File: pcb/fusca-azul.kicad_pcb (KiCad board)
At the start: 2 copper layers, 59 x 67.5 mm, 12 parts, among them J3 HC-SR04, J4 L298N Logic Jumpers, J5 HC-SR04, J6 HC-SR04, U2 ESP32 - HW-394

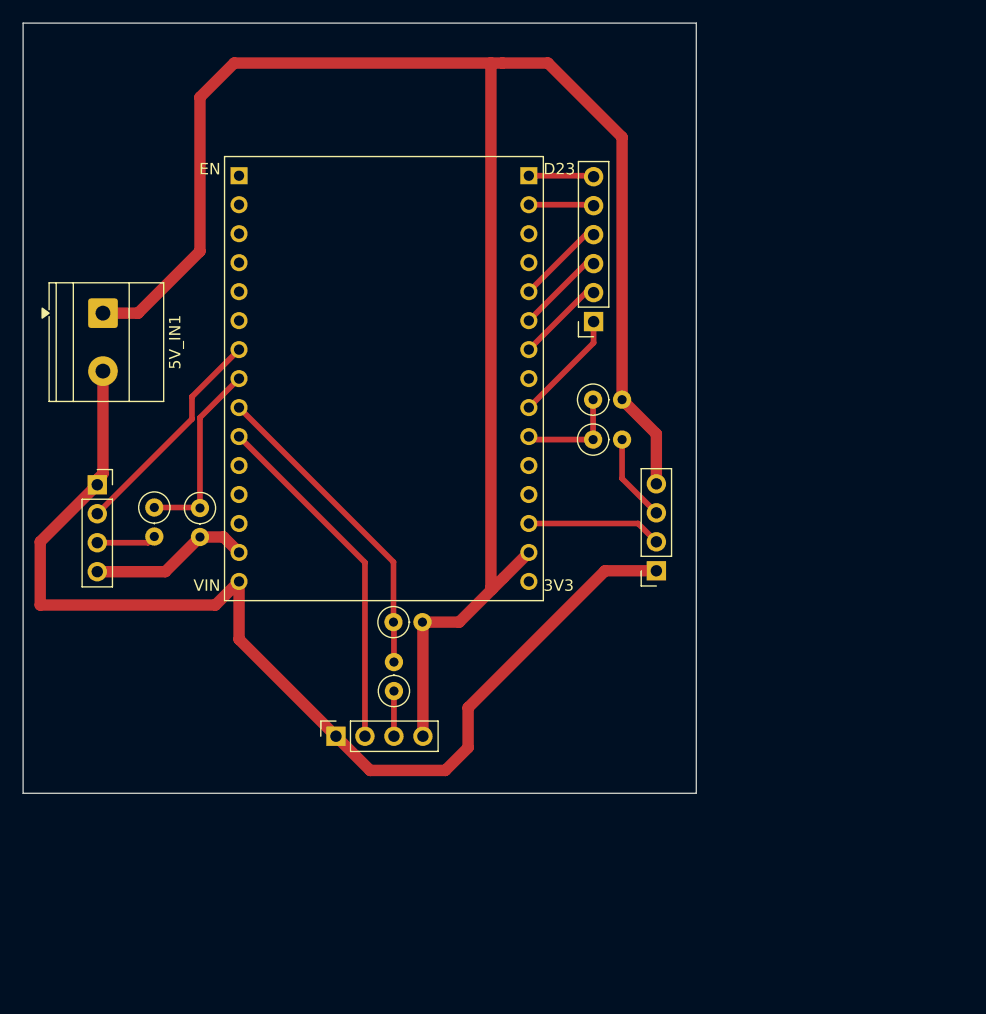
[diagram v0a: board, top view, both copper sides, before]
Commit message: finaliza pcb
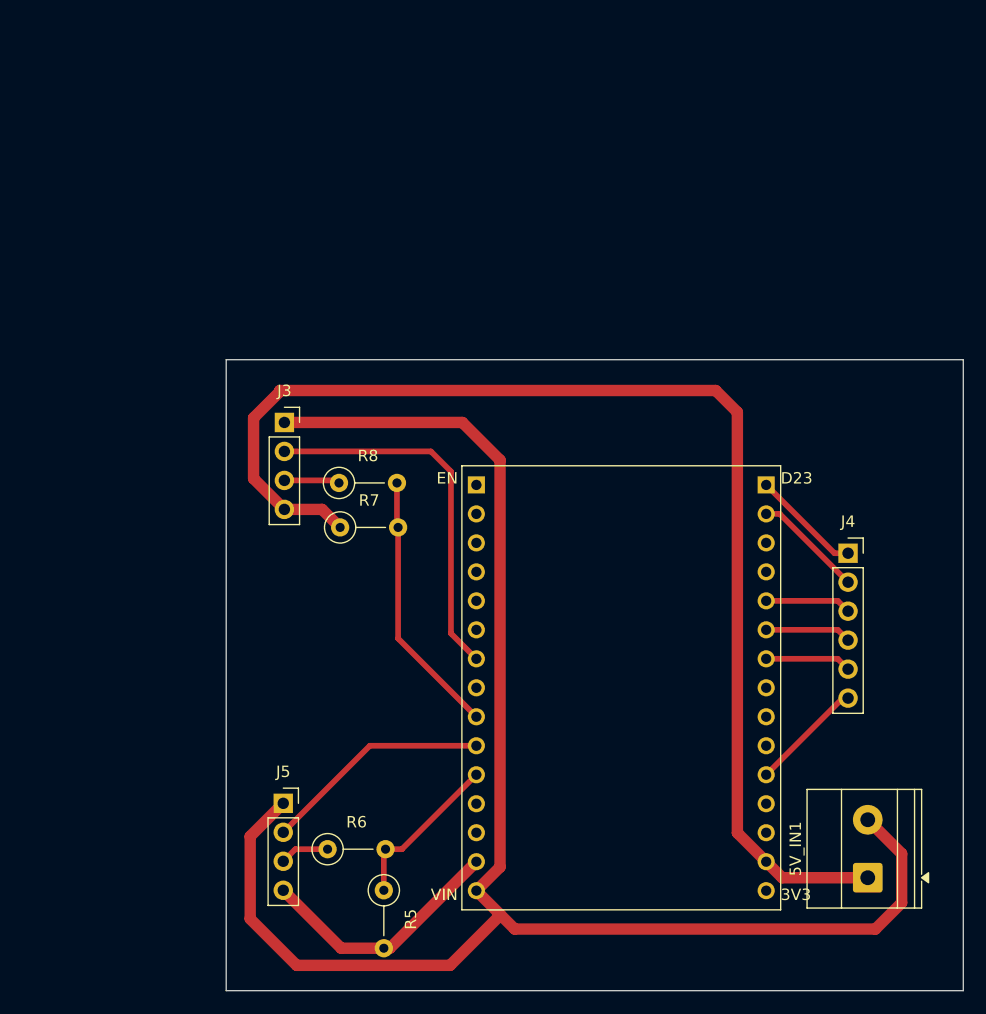
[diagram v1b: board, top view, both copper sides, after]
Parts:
- removed J6: HC-SR04, Connector_PinSocket_2.54mm:PinSocket_1x04_P2.54mm_Vertical
- removed R3: 2k, Resistor_THT:R_Axial_DIN0207_L6.3mm_D2.5mm_P2.54mm_Vertical
- removed R4: 1k, Resistor_THT:R_Axial_DIN0207_L6.3mm_D2.5mm_P2.54mm_Vertical
- R5, R6, R7, R8: footprint Resistor_THT:R_Axial_DIN0207_L6.3mm_D2.5mm_P2.54mm_Vertical -> Resistor_THT:R_Axial_DIN0207_L6.3mm_D2.5mm_P5.08mm_Vertical
- moved 5V_IN1 83.3 mm to (154.0, 122.4), turned to 90 degrees
- moved R5 37.2 mm to (111.6, 123.5)
- moved U2 34.2 mm to (119.7, 88.0)
- moved R6 33.6 mm to (106.7, 119.9), turned to 0 degrees
- moved J5 32.3 mm to (102.8, 115.9)
- moved J4 30.2 mm to (152.3, 94.0), turned to 0 degrees
- moved J3 27.9 mm to (102.9, 82.5), turned to 0 degrees
- moved R8 18.9 mm to (107.7, 87.8), turned to 0 degrees
- moved R7 9.53 mm to (107.8, 91.7)
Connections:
- R5 pad 1: Net-(U2-D25) -> Net-(U2-D14)
- R6 pad 1: Net-(U2-D25) -> Net-(J5-Echo)
- R6 pad 2: Net-(J5-Echo) -> Net-(U2-D14)
- R7 pad 1: Net-(U2-D26) -> GND
- R7 pad 2: GND -> Net-(U2-D26)
- U2 pad 18: Net-(J6-Trig) -> unconnected-(U2-D15-Pad18)
- U2 pad 20: unconnected-(U2-D4-Pad20) -> Net-(J4-ENB)
- U2 pad 21: Net-(U2-RX2) -> unconnected-(U2-RX2-Pad21)
- U2 pad 22: Net-(J4-ENA) -> unconnected-(U2-TX2-Pad22)
- U2 pad 24: Net-(J4-IN_1) -> Net-(J4-IN_4)
- U2 pad 25: Net-(J4-IN_2) -> Net-(J4-IN_3)
- U2 pad 26: Net-(J4-IN_3) -> Net-(J4-IN_2)
- U2 pad 29: Net-(J4-IN_4) -> Net-(J4-IN_1)
- U2 pad 30: Net-(J4-ENB) -> Net-(J4-ENA)
- U2 pad 5: unconnected-(U2-D14-Pad5) -> Net-(U2-D14)
- U2 pad 6: Net-(J3-Trig) -> Net-(J5-Trig)
- U2 pad 8: Net-(U2-D25) -> unconnected-(U2-D25-Pad8)
- U2 pad 9: Net-(J5-Trig) -> Net-(J3-Trig)
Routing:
- net GND: track 179.1 -> 131.0 mm
- net +5V: track 96.8 -> 143.8 mm
- net Net-(U2-D25): track 16.8 -> 0.00 mm
- net Net-(U2-D14): track 0.00 -> 14.3 mm
- net Net-(J6-Trig): track 11.8 -> 0.00 mm
- net Net-(U2-RX2): track 9.24 -> 0.00 mm
- net Net-(J6-Echo): track 7.66 -> 0.00 mm
- net Net-(U2-D26): track 27.9 -> 23.4 mm
- net Net-(J4-ENB): track 5.71 -> 9.96 mm
- net Net-(J4-IN_1): track 7.74 -> 9.65 mm
- net Net-(J4-IN_4): track 5.71 -> 7.55 mm
- net Net-(J3-Trig): track 30.8 -> 32.7 mm
- net Net-(J3-Echo): track 3.96 -> 4.88 mm
- net Net-(J5-Echo): track 5.23 -> 4.32 mm
- net Net-(J5-Trig): track 19.5 -> 20.1 mm
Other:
- board size 59 x 67.5 mm -> 64.6 x 55.3 mm
